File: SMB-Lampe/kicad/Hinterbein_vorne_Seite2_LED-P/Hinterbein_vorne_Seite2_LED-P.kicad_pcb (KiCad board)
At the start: 2 copper layers, 10.7 x 29.2 mm, 5 parts

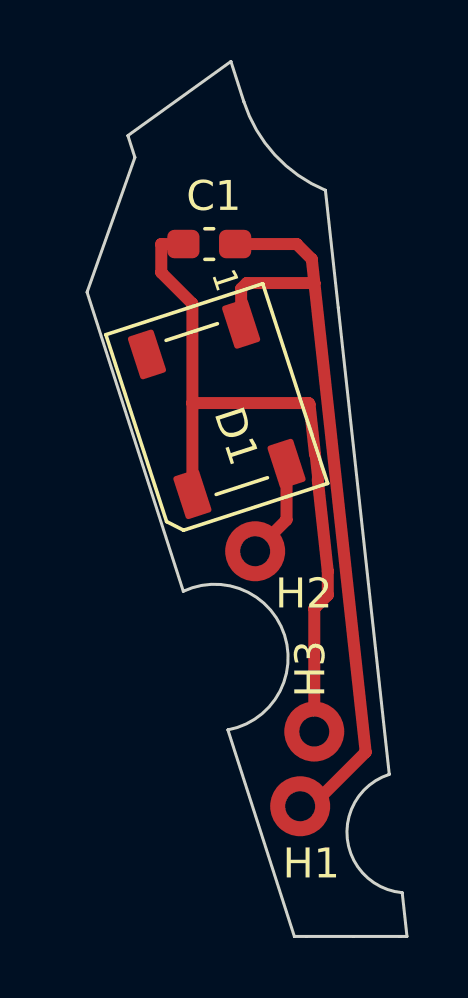
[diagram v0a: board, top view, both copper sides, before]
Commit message: Alle Platinen sind fertig zur Fertigung
Aus diesem Stand folgt das erste fertig leuchtende Pferd
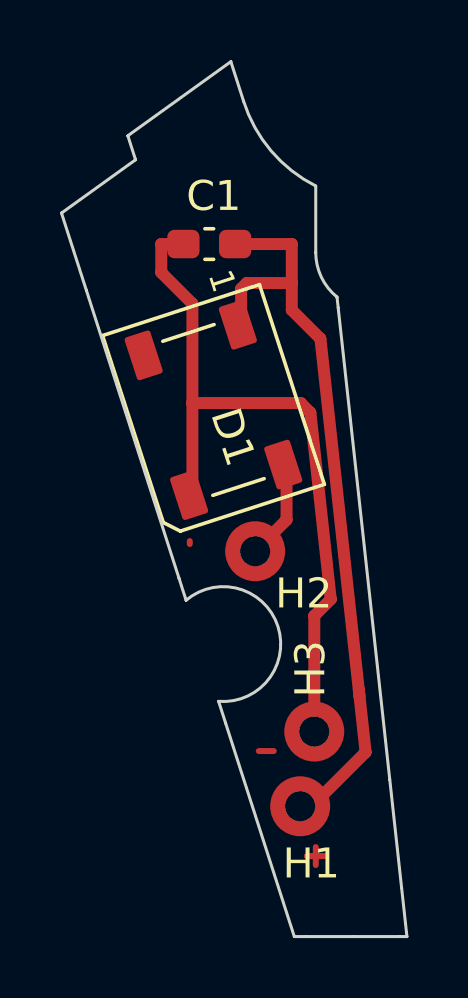
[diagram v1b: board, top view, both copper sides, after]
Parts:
- moved D1 0.11 mm to (151.5, 99.6)
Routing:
- net /+5V_IN_Hinterbein_vorne_Seite1: track 25.5 -> 25.0 mm
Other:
- board size 10.7 x 29.2 mm -> 11.5 x 29.2 mm
